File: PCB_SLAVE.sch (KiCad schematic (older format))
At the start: 44 parts, among them J1 RGB, J10 DHT, J2 POWER_12V, J3 MOTOR_DC, J4 LED_OUT, J7 MOTOR, J8 zigbee, J9 DAT, K1 G5LE-1, Q1 2SC1815, Q2 IRF540N, Q3 2SC1815, SW1 NGUON, SW2 SW_Push, SW3 SW_Push, U1 PC817, U2 LM2576HVS-AJD

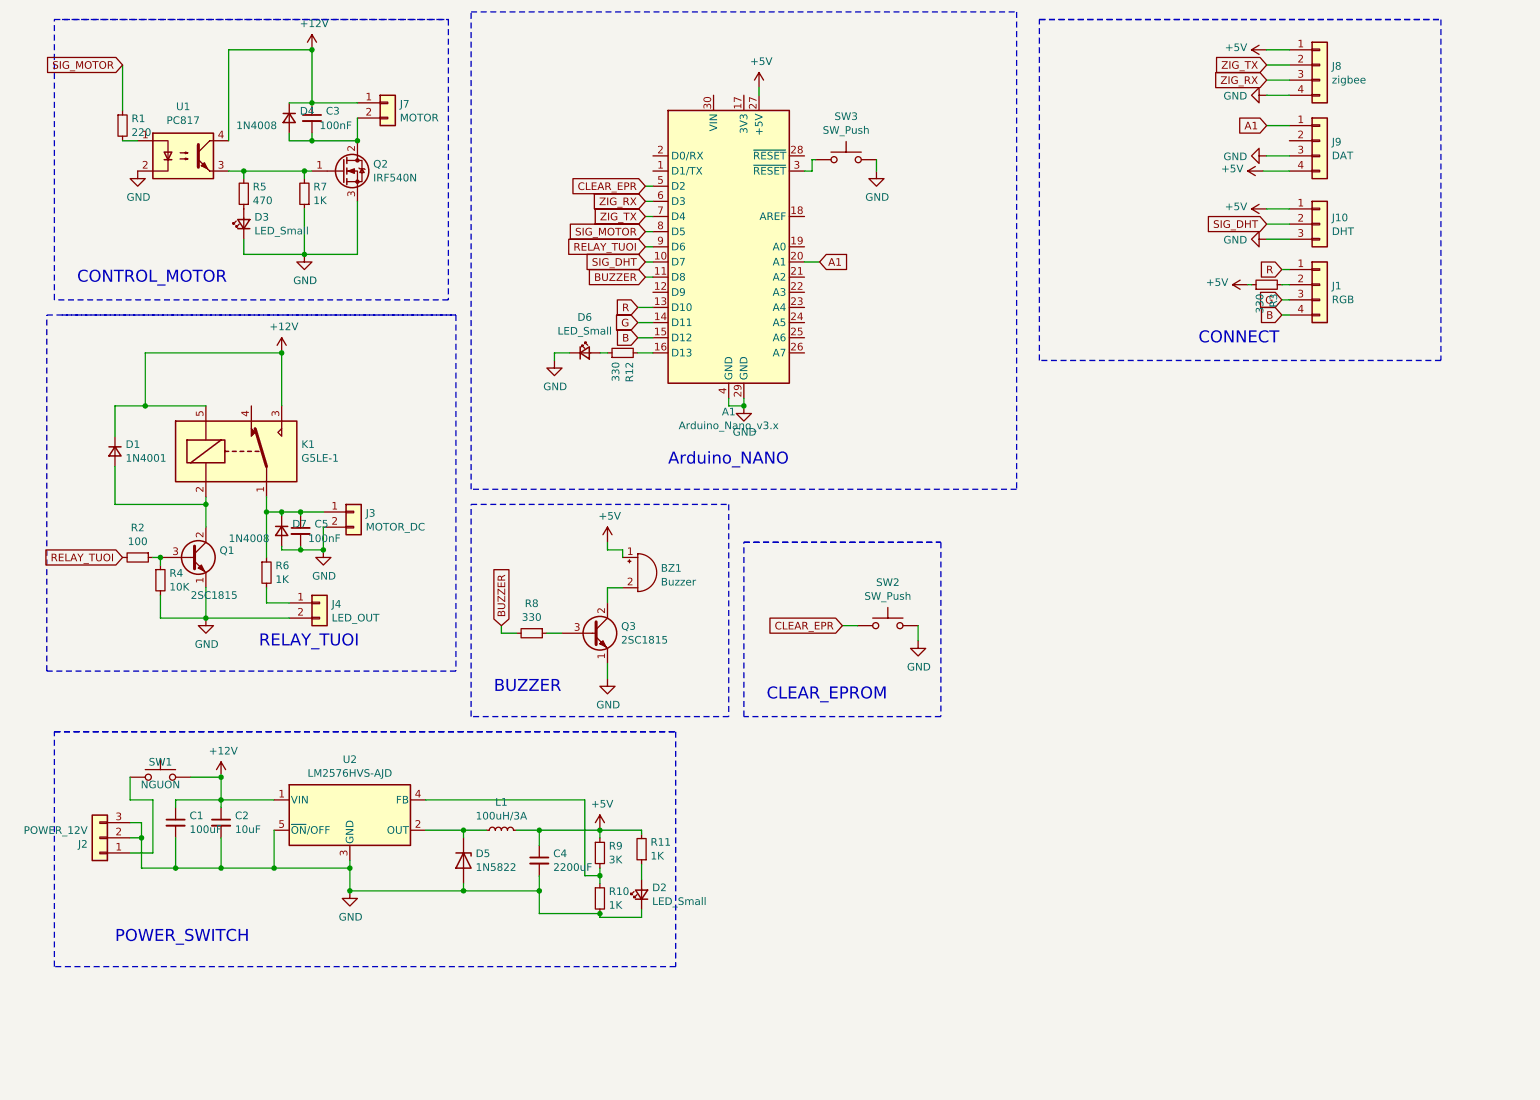
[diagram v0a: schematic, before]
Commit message: edit
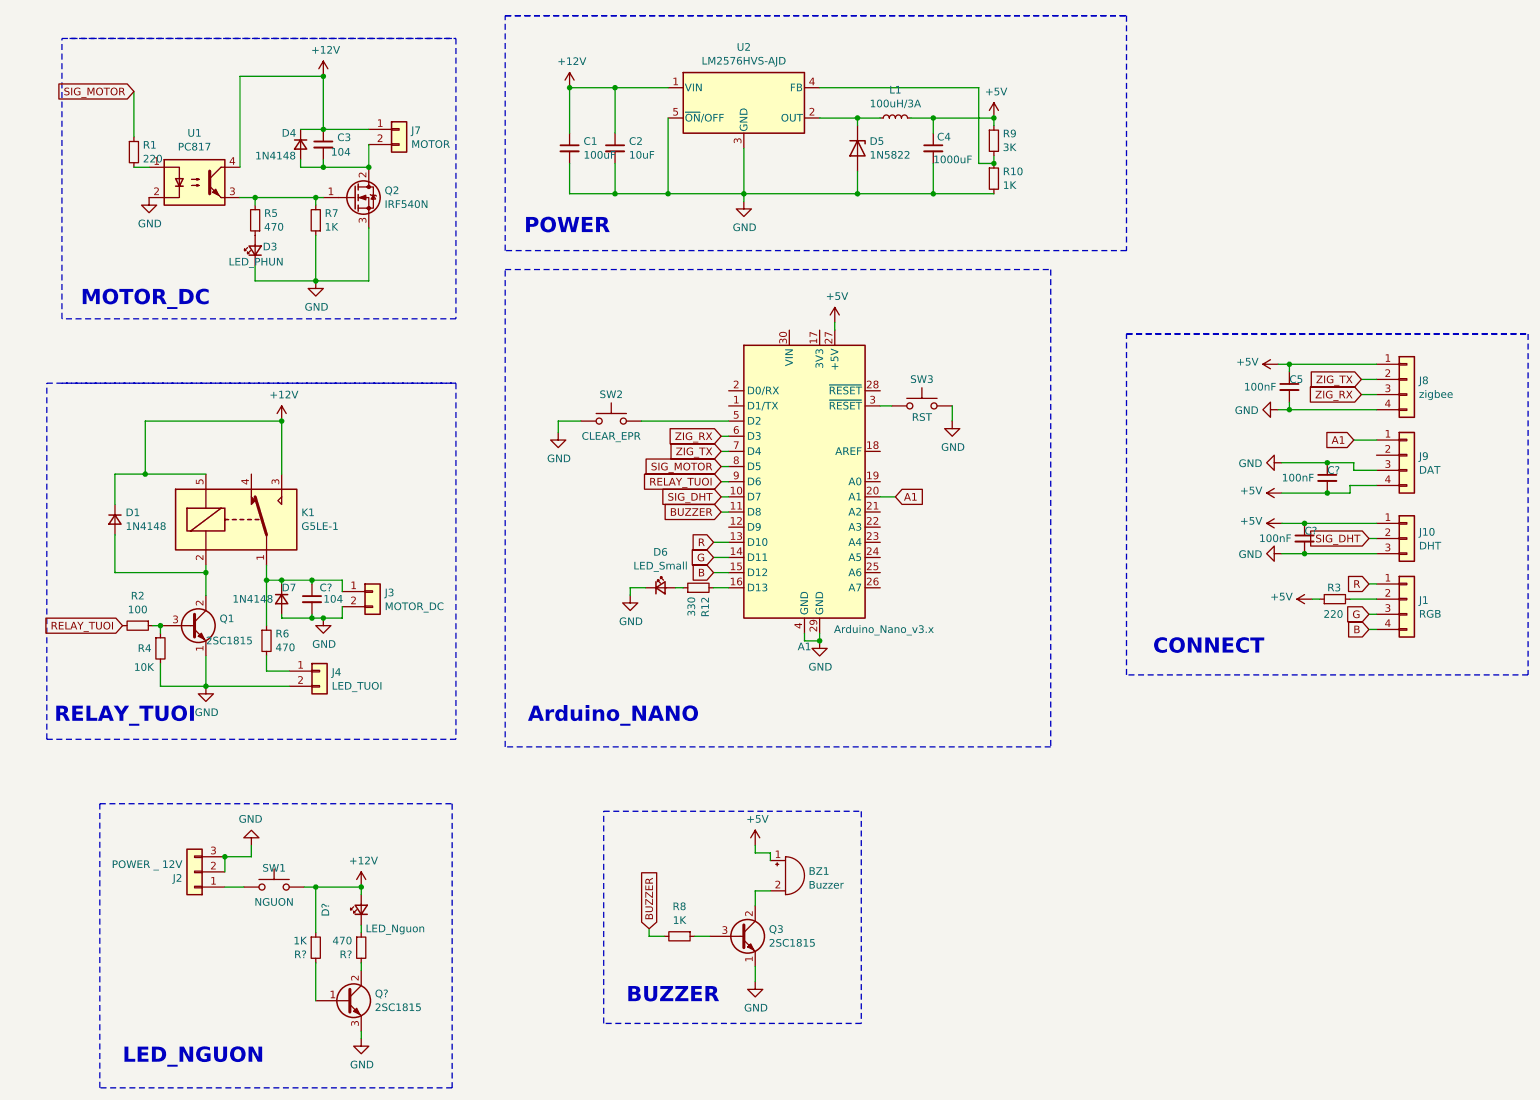
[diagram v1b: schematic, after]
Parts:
- removed D2: LED_Small, Connector_PinHeader_2.54mm:PinHeader_1x02_P2.54mm_Vertical, symbol Device:LED_Small
- removed R11: 1K, Resistor_THT:R_Axial_DIN0207_L6.3mm_D2.5mm_P10.16mm_Horizontal, symbol Device:R_Small
- added C? (x2): 100nF, Capacitor_THT:CP_Radial_D5.0mm_P2.50mm, symbol Device:C_Small
- added C?: 104, Capacitor_THT:CP_Radial_D5.0mm_P2.50mm, symbol Device:C_Small
- added D?: LED_Nguon, LED_THT:LED_D3.0mm, symbol Device:LED_Small
- added Q?: 2SC1815, symbol Device:Q_NPN_BCE
- added R?: 1K, Resistor_THT:R_Axial_DIN0309_L9.0mm_D3.2mm_P15.24mm_Horizontal, symbol Device:R_Small
- added R?: 470, Resistor_THT:R_Axial_DIN0309_L9.0mm_D3.2mm_P15.24mm_Horizontal, symbol Device:R_Small
- C3: value 100nF -> 104
- C4: value 2200uF -> 1000uF
- D1: value 1N4001 -> 1N4148
- D3: value LED_Small -> LED_PHUN
- D4, D7: value 1N4008 -> 1N4148
- J2: value POWER_12V -> POWER _ 12V
- J4: value LED_OUT -> LED_TUOI
- R3: value 330 -> 220
- R6: value 1K -> 470
- R8: value 330 -> 1K
- SW2: value SW_Push -> CLEAR_EPR
- SW3: value SW_Push -> RST
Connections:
- net +12V: now also D?.2 (A), R?.1
- net +5V: now also C5.1, C?.1, C?.2
- net GND: now also SW2.1, C?.1, C?.2, C?.2, Q?.3 (E); no longer SW2.2
- net at D7.1 (K), J3.1 (Pin_1), K1.1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: now also C?.1; no longer C5.1
- net CLEAR_EPR: no longer names the net of A1.5 (D2)
- net CLEAR_EPR: now also SW2.2; no longer SW2.1
- new net: Q?.1 (B), R?.2
- new net: Q?.2 (C), R?.2
- new net: D?.1 (K), R?.1
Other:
- note added: "LED_NGUON\n"
- note added: "MOTOR_DC\n"
- note added: "POWER\n"
- note removed: "CLEAR_EPROM"
- note removed: "CONTROL_MOTOR"
- note removed: "POWER_SWITCH\n"
- moved on the sheet: A1, BZ1, C1, C2, C3, C4, C5, D1, D3, D4, D5, D6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
